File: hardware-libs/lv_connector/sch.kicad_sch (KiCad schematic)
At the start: 1 part, among them J1 212528-0600

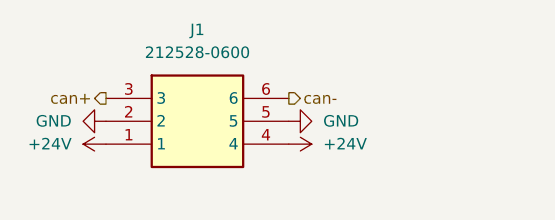
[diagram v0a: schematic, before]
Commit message: Update connector
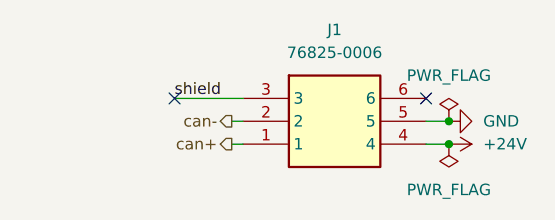
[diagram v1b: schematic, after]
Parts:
- removed J1: 212528-0600, 212528-0600:212528-06YY_1, symbol 212528-0600:212528-0600
- added J1: 76825-0006, 768250006, symbol 76825-0006:76825-0006
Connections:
- net +24V: now also J1.4
- net GND: now also J1.5
- net can+: now also J1.1
- net can-: now also J1.2
- new net shield: J1.3
- no-connect marks 0 -> 2
